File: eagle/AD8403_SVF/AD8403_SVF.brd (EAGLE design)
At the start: 70.8 x 45.7 mm, 30 parts, among them IC1 AD8403-DIP24, IC2 NJM2732, IC3 NJM2732

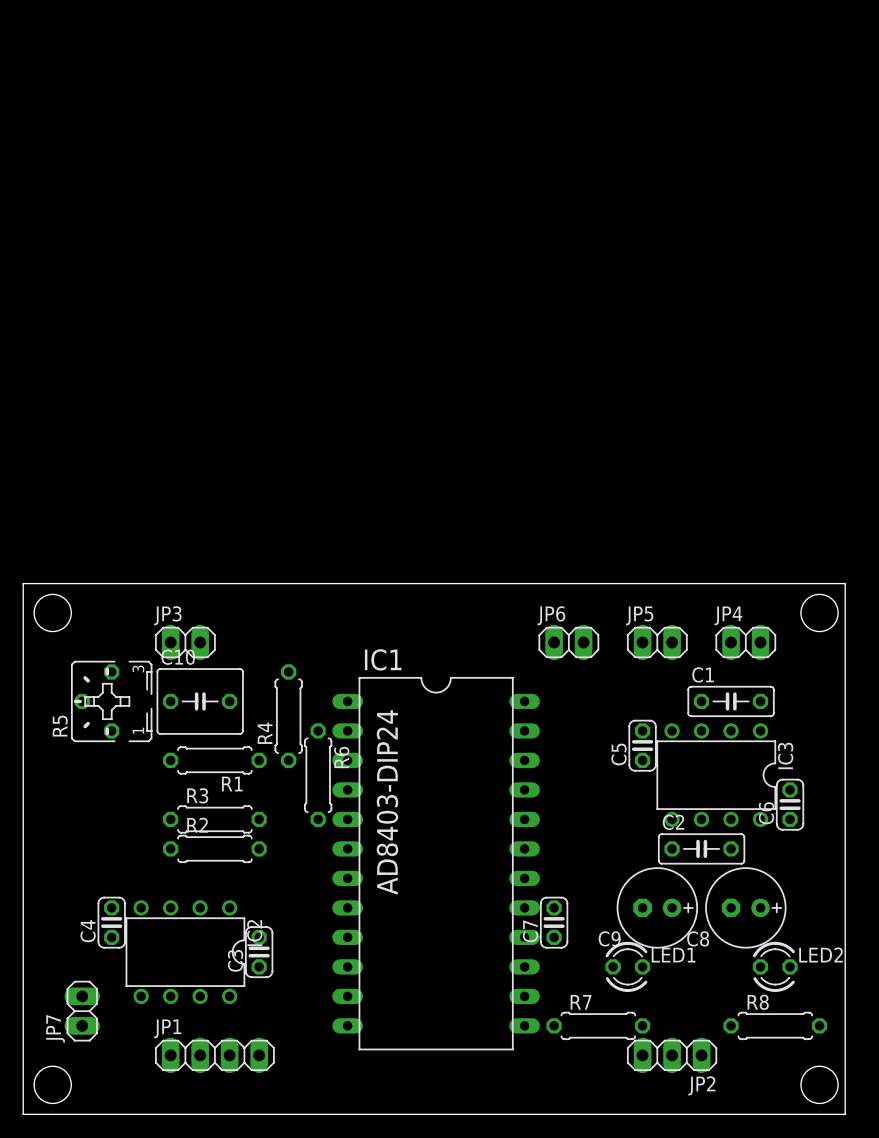
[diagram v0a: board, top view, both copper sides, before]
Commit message: Update: eagle files
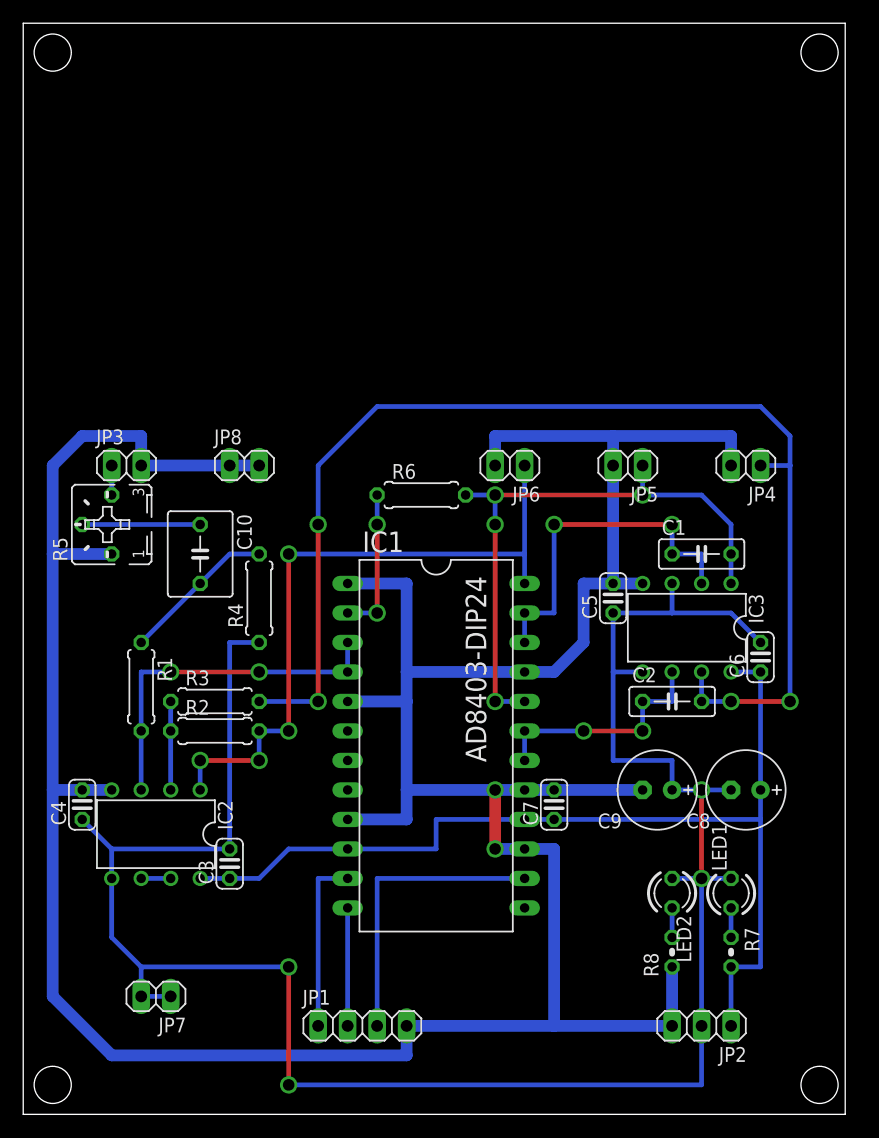
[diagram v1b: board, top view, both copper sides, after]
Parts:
- added JP8: GND, pinhead:1X02
- R7, R8: device rcl:0207/7 -> rcl:0204V
- moved R6 25.7 mm to (34.3, 53.3), turned to 0 degrees
- moved JP3 16.1 mm to (8.89, 55.9)
- moved JP6 16.1 mm to (41.9, 55.9), turned to 180 degrees
- moved JP5 15.5 mm to (52.1, 55.9), turned to 180 degrees
- moved JP4 15.2 mm to (62.2, 55.9), turned to 180 degrees
- moved R5 15.2 mm to (7.62, 50.8)
- moved R7 13.1 mm to (61.0, 14.0), turned to 270 degrees
- moved C2 13.0 mm to (55.9, 35.6)
- moved C5 13.0 mm to (50.8, 44.5)
- moved JP1 13.0 mm to (29.2, 7.62)
- moved C1 13.0 mm to (58.4, 48.3)
- moved C6 13.0 mm to (63.5, 39.4)
- moved IC3 13.0 mm to (57.1, 41.9)
- moved C10 12.7 mm to (15.2, 48.3), turned to 270 degrees
- moved LED1 10.9 mm to (61.0, 19.1), turned to 90 degrees
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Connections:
- removed net N$15: LED1.K, R7.2
- new net N$13: LED1.A, R7.1
- net +5V: now also R7.2; no longer LED1.A
- net GND: now also JP4.2, JP5.2, JP6.2, JP8.1, JP8.2
- net VCC/2: now also LED1.K; no longer JP4.2, JP5.2, JP6.2, R7.1
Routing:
- net GND: track 0.00 -> 286.1 mm, vias 0 -> 2
- net VCC/2: track 0.00 -> 183.5 mm, vias 0 -> 4
- net N$9: track 0.00 -> 104.8 mm, vias 0 -> 4
- net +5V: track 0.00 -> 87.4 mm
- net N$5: track 0.00 -> 58.4 mm, vias 0 -> 4
- net N$10: track 0.00 -> 51.9 mm, vias 0 -> 4
- net N$3: track 0.00 -> 30.5 mm, vias 0 -> 2
- net N$7: track 0.00 -> 30.5 mm, vias 0 -> 2
- net SCK: track 0.00 -> 25.4 mm
- net N$6: track 0.00 -> 20.3 mm, vias 0 -> 2
- net !CS: track 0.00 -> 15.2 mm
- net N$11: track 0.00 -> 13.3 mm
- net N$12: track 0.00 -> 12.7 mm, vias 0 -> 2
- net N$2: track 0.00 -> 10.2 mm
- net MOSI: track 0.00 -> 10.2 mm
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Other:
- board size 70.8 x 45.7 mm -> 70.8 x 94 mm
